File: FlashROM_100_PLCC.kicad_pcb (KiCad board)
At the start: 2 copper layers, 17.8 x 35.6 mm, 6 parts, among them J1 LH535618 DIP LEGS, U1 29F010

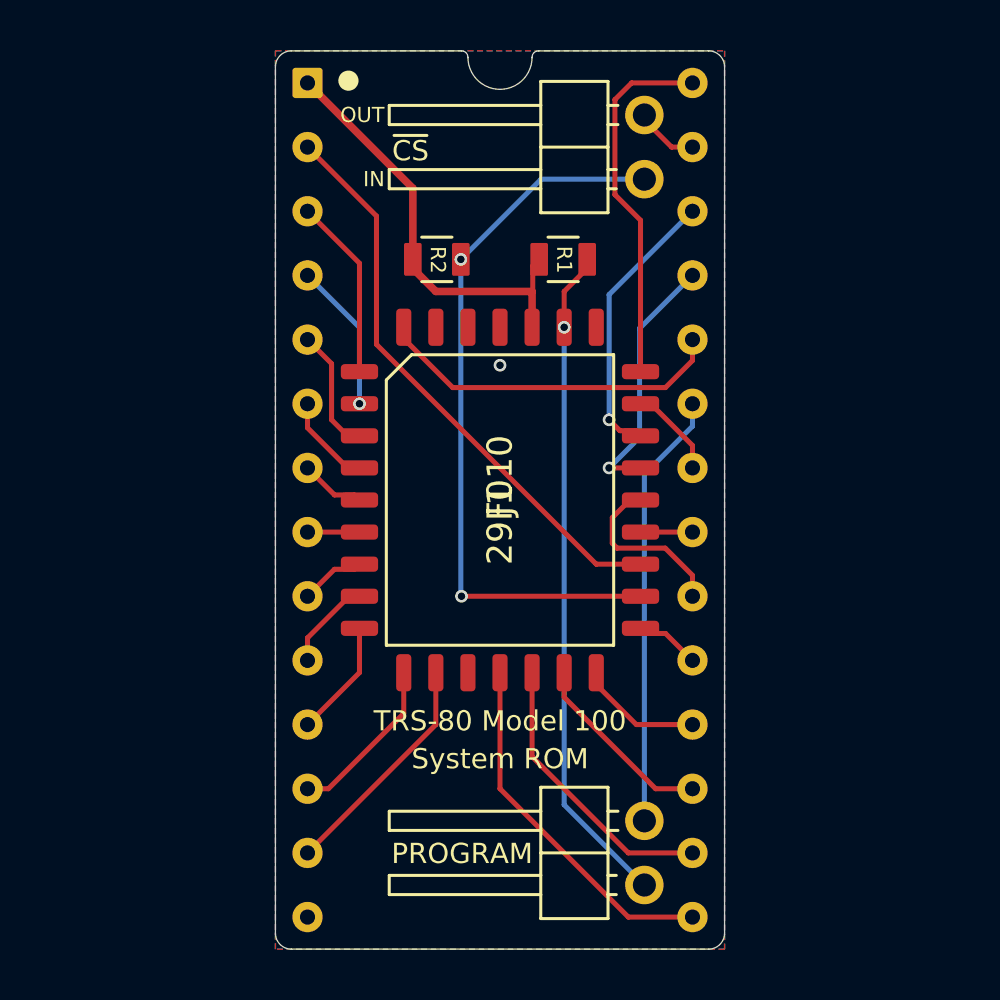
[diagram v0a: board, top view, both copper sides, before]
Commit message: various minor cleanups
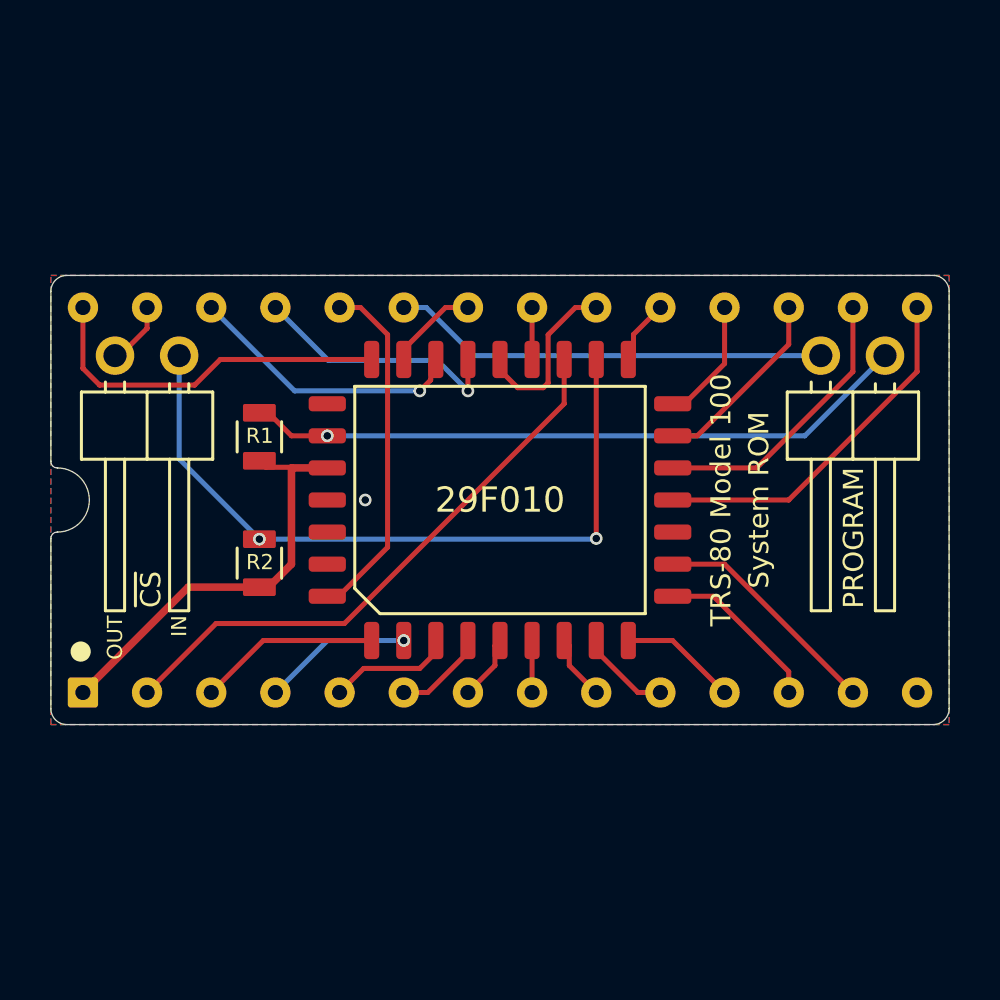
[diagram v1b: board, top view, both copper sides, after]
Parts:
- JP1: value ~CS~ breakout -> ~{CS} breakout
- moved JP2 23.0 mm to (165.2, 94.3), turned to -90 degrees
- moved JP1 19.7 mm to (137.3, 94.3), turned to -90 degrees
- moved R1 13.9 mm to (140.5, 97.5), turned to -90 degrees
- moved R2 13.9 mm to (140.5, 102.5), turned to -90 degrees
- turned J1 to 90 degrees
- turned U1 to 90 degrees
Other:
- board size 17.8 x 35.6 mm -> 35.6 x 17.8 mm
- board text added: "${COMMENT2} ${TITLE} ${REVISION}"
- board text added: "R1,R2: ${00000000-0000-0000-0000-0000604ac043:VALUE} Legs: TE 1544210"
- board text added: "REX_Classic main ROM support: ~{CS}_OUT to REX TP1 to boot from REX main rom ~{CS}_OUT to ~{CS}_IN to boot from internal main rom"
- board text removed: "Connect ~{CS} OUT to REX TP1. Leave ~{CS} IN unconnected."
- board text removed: "If REX is later removed, connect ~{CS} OUT to ~{CS} IN."
- board text removed: "Install a shunt on ~{CS}, or, install wires as above,"
- board text removed: "Legs: TE 1544210"
- board text removed: "R1, R2: 47k"
- board text removed: "REX can then be added later without disassembling."
- board text removed: "Run 2 wires from ~{CS} IN & ~{CS} OUT to Option ROM compartment."
- board text removed: "To use REX Main ROM feature:"
- board text removed: "To use without REX:"
- board text removed: "and connect them to each other in the Option ROM compartment."
